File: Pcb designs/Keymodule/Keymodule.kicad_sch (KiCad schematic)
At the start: 107 parts, among them J1 Conn_01x01, J11 USB connect, J2 Conn_01x01, J3 Conn_01x03, J4 Conn_01x01, J5 Conn_01x01, J6 Conn_01x03, U1 RP2040, U2 SN74LV1T34DBV, U3 AMS1117-3.3, U4 W25Q128JVS, Y1 ABM8-272-T3

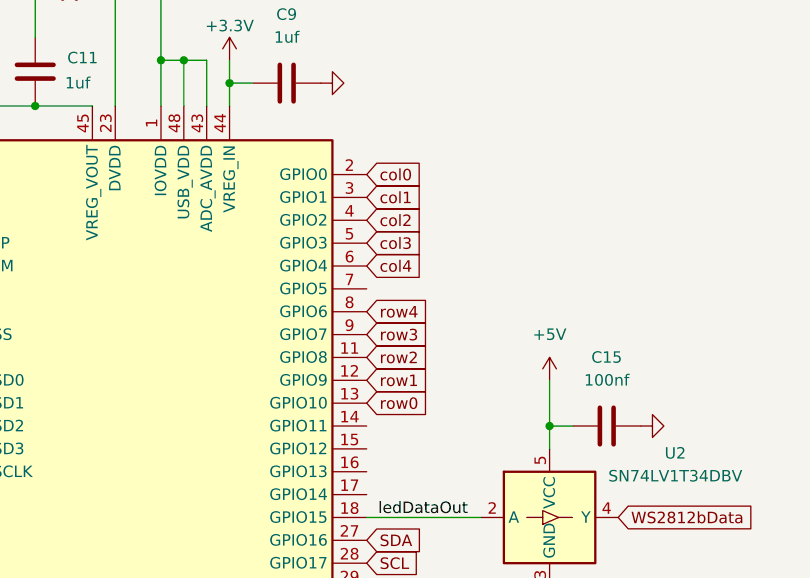
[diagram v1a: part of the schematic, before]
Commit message: Ihope this is the one
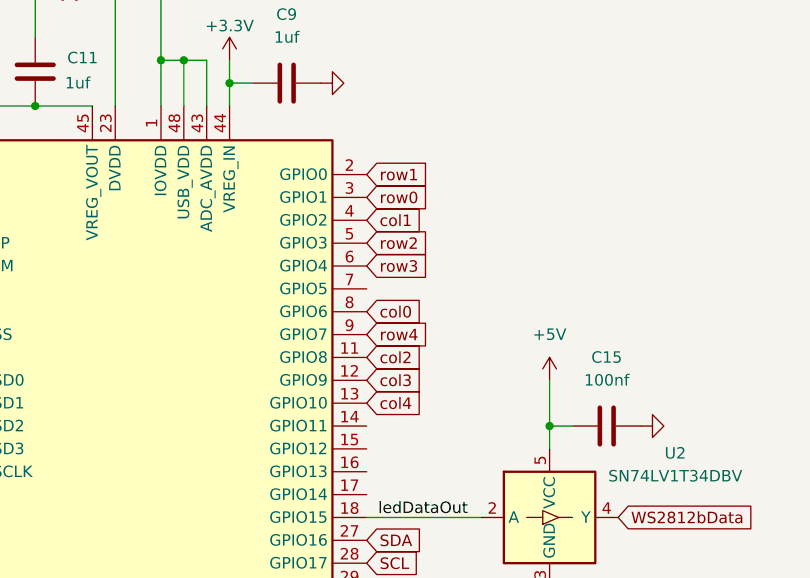
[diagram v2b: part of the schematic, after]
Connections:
- net col0: now also U1.8 (GPIO6); no longer U1.2 (GPIO0)
- net col1: now also U1.4 (GPIO2); no longer U1.3 (GPIO1)
- net col2: now also U1.11 (GPIO8); no longer U1.4 (GPIO2)
- net col3: now also U1.12 (GPIO9); no longer U1.5 (GPIO3)
- net col4: now also U1.13 (GPIO10); no longer U1.6 (GPIO4)
- net row0: now also U1.3 (GPIO1); no longer U1.13 (GPIO10)
- net row1: now also U1.2 (GPIO0); no longer U1.12 (GPIO9)
- net row2: now also U1.5 (GPIO3); no longer U1.11 (GPIO8)
- net row3: now also U1.6 (GPIO4); no longer U1.9 (GPIO7)
- net row4: now also U1.9 (GPIO7); no longer U1.8 (GPIO6)
